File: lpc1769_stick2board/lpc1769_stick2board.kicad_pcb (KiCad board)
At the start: 2 copper layers, 63.5 x 97.5 mm, 14 parts, among them J1 Conn_01x27, J2 Conn_01x27, J3 Conn_02x10_Odd_Even, M3 MountingHole_3.2mm_M3, U1 LPCXpresso_LPC1769_revB

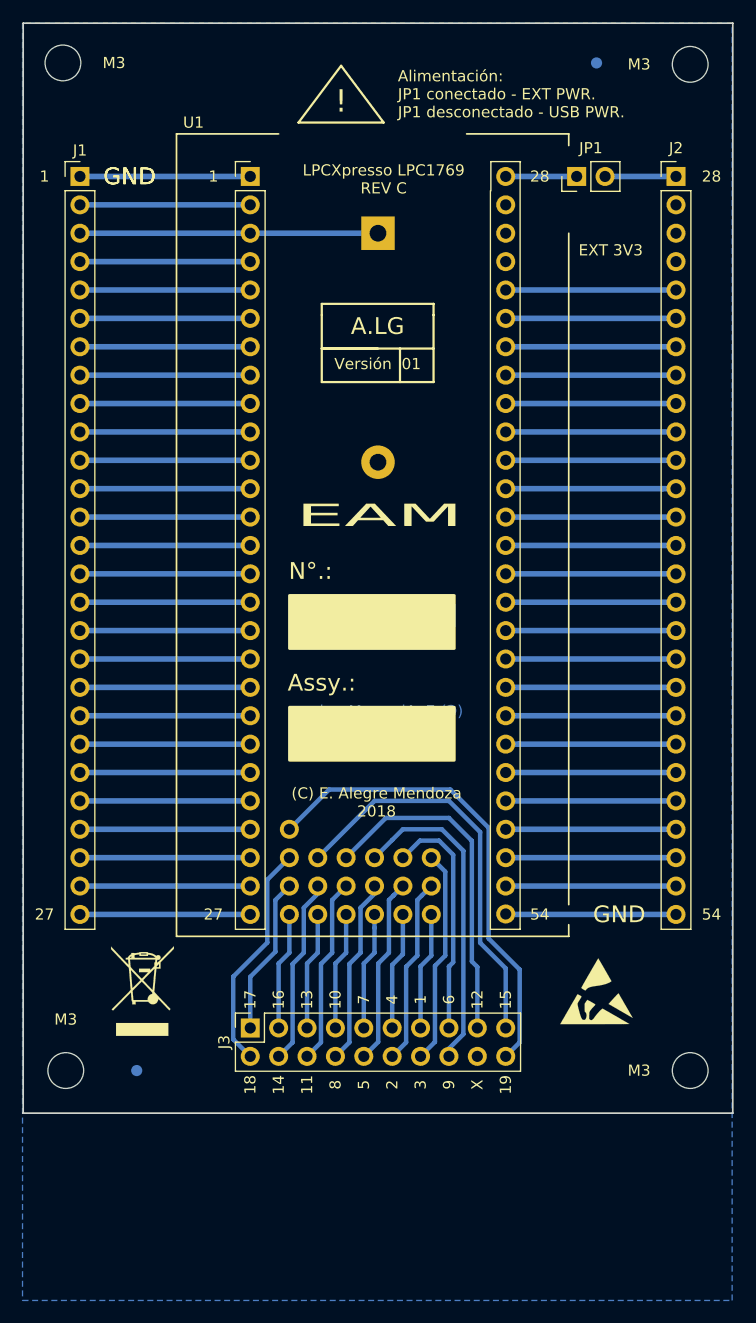
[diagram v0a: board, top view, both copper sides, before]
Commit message: PLACA TERMINADA. LISTA PARA PLANCHAR
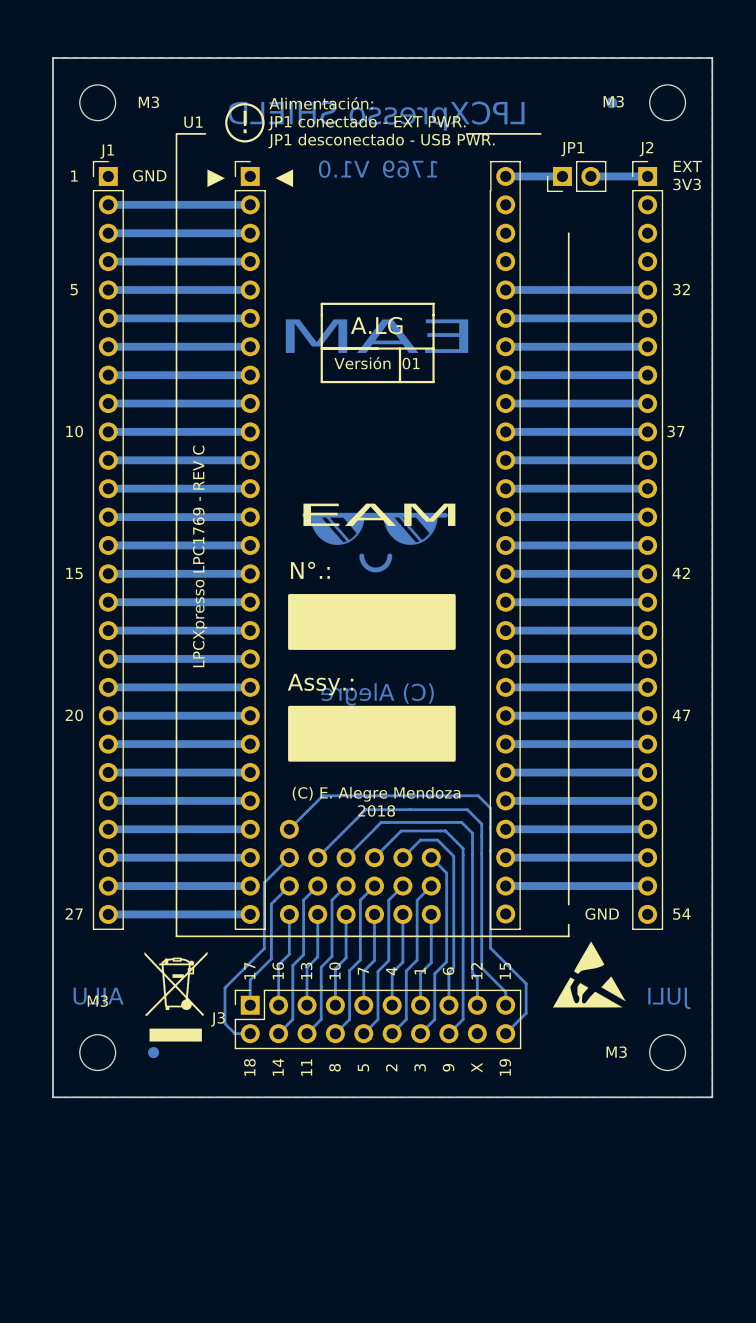
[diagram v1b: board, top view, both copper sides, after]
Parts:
- removed BT1: Battery_Cell, Battery_Holders:Keystone_106_1x20mm-CoinCell
- added G***: LOGO, footprints:emoji_6, B.Cu at (147.8, 102.4)
- moved M3 4.73 mm to (123.0, 63.0)
- moved M3 3.99 mm to (174.0, 63.0)
- moved F1 3.81 mm to (169.0, 63.0)
- moved M3 3.28 mm to (123.0, 148.0)
- moved REF*** 3.04 mm to (130.0, 143.0)
- moved M3 2.58 mm to (174.0, 148.0)
- moved J2 2.54 mm to (172.2, 69.6)
- moved J1 2.54 mm to (124.0, 69.6)
- moved F2 2.20 mm to (128.0, 148.0)
- moved J3 2.03 mm to (136.7, 143.8)
- moved REF*** 1.63 mm to (167.0, 141.0)
- moved JP1 1.27 mm to (164.6, 69.6)
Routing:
- net GND: track 30.5 -> 0.00 mm
- net Net-(J1-Pad3): track 26.7 -> 12.7 mm
- net Net-(J2-Pad9): track 15.2 -> 12.7 mm
- net Net-(J2-Pad8): track 15.2 -> 12.7 mm
- net Net-(J2-Pad7): track 15.2 -> 12.7 mm
- net Net-(J2-Pad6): track 15.2 -> 12.7 mm
- net Net-(J2-Pad5): track 15.2 -> 12.7 mm
- net Net-(J2-Pad26): track 15.2 -> 12.7 mm
- net Net-(J2-Pad25): track 15.2 -> 12.7 mm
- net Net-(J2-Pad24): track 15.2 -> 12.7 mm
- net Net-(J2-Pad23): track 15.2 -> 12.7 mm
- net Net-(J2-Pad22): track 15.2 -> 12.7 mm
- net Net-(J2-Pad21): track 15.2 -> 12.7 mm
- net Net-(J2-Pad20): track 15.2 -> 12.7 mm
- net Net-(J2-Pad19): track 15.2 -> 12.7 mm
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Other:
- board size 63.5 x 97.5 mm -> 59 x 93 mm
- board text added: "(C) Alegre Mendoza E. 2018"
- board text added: "1769"
- board text added: "20"
- board text added: "32"
- board text added: "37"
- board text added: "42"
- board text added: "47"
- board text added: "AILU"
- board text added: "JULI"
- board text added: "LPCXpresso LPC1769 - REV C"
- board text added: "LPCXpresso SHIELD"
- board text added: "V1.0"
- board text added: "▶"
- board text removed: "28"
- board text removed: "EZEQUIEL ALEGRE"
- board text removed: "LPCXpresso LPC1769 REV C"
